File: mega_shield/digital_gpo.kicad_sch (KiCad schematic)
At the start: 26 parts, among them J23 1803277, J24 1803277, Q25 MMBT3904, Q26 MMBT3906, Q27 MMBT3904, Q28 MMBT3906, Q29 AO4486, Q30 AO4486, U26 ADuM1200

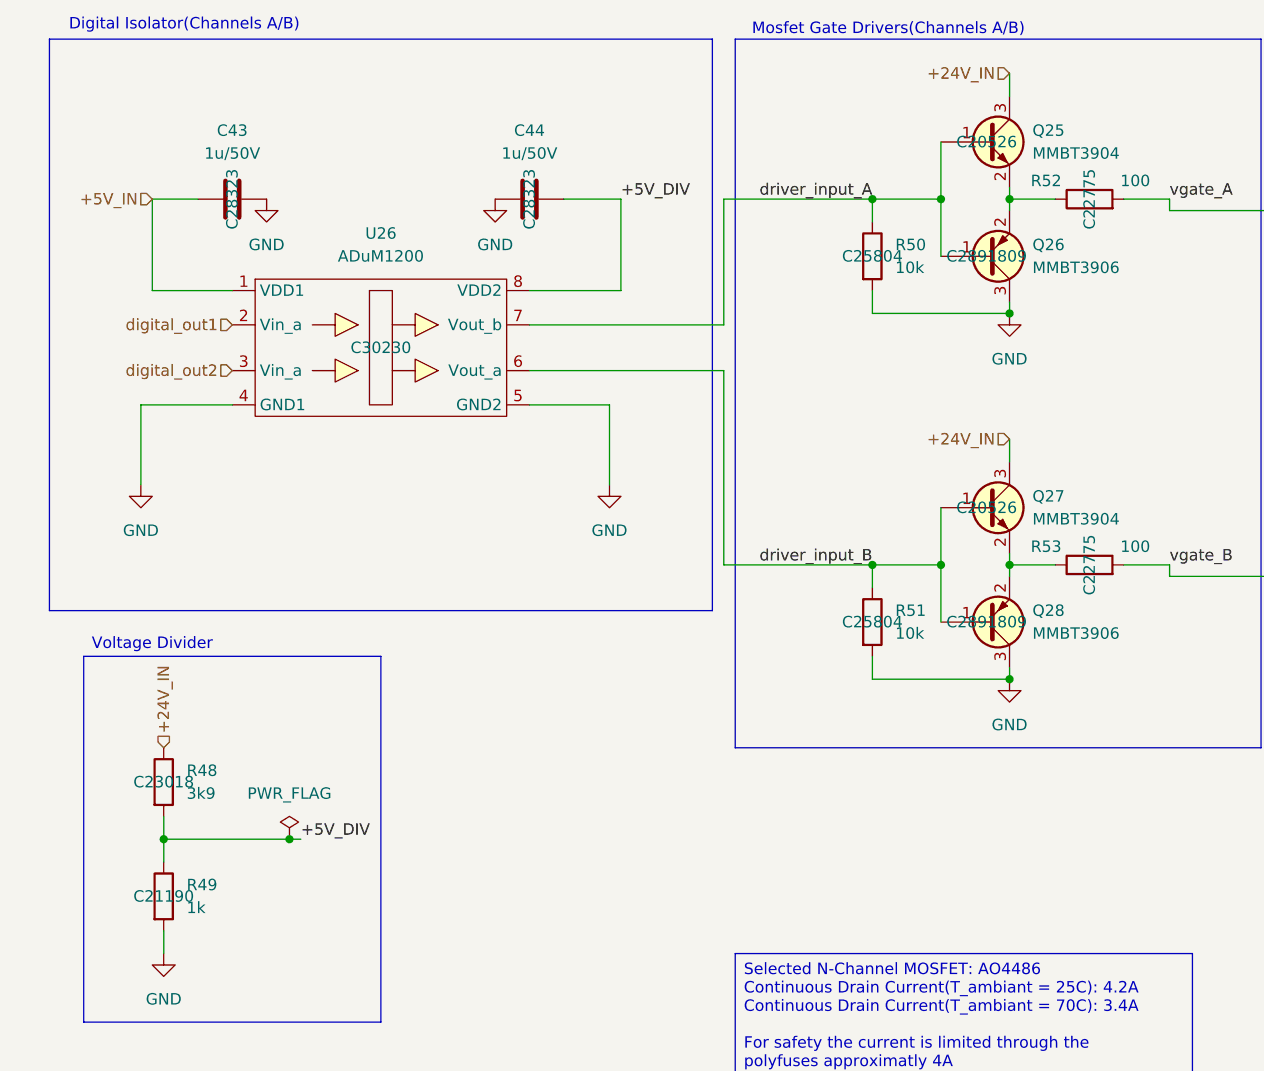
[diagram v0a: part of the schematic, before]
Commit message: mega_shield, updated multiple resistors and added comments.
+ Updated optoisolator resistor value --> 15k for better protection.
+ Changed all resistors to 0805 footprints
+ Swapped out expensive values to standardized E24/E96.
+ Updated jlcpcb numbers for all resistors.
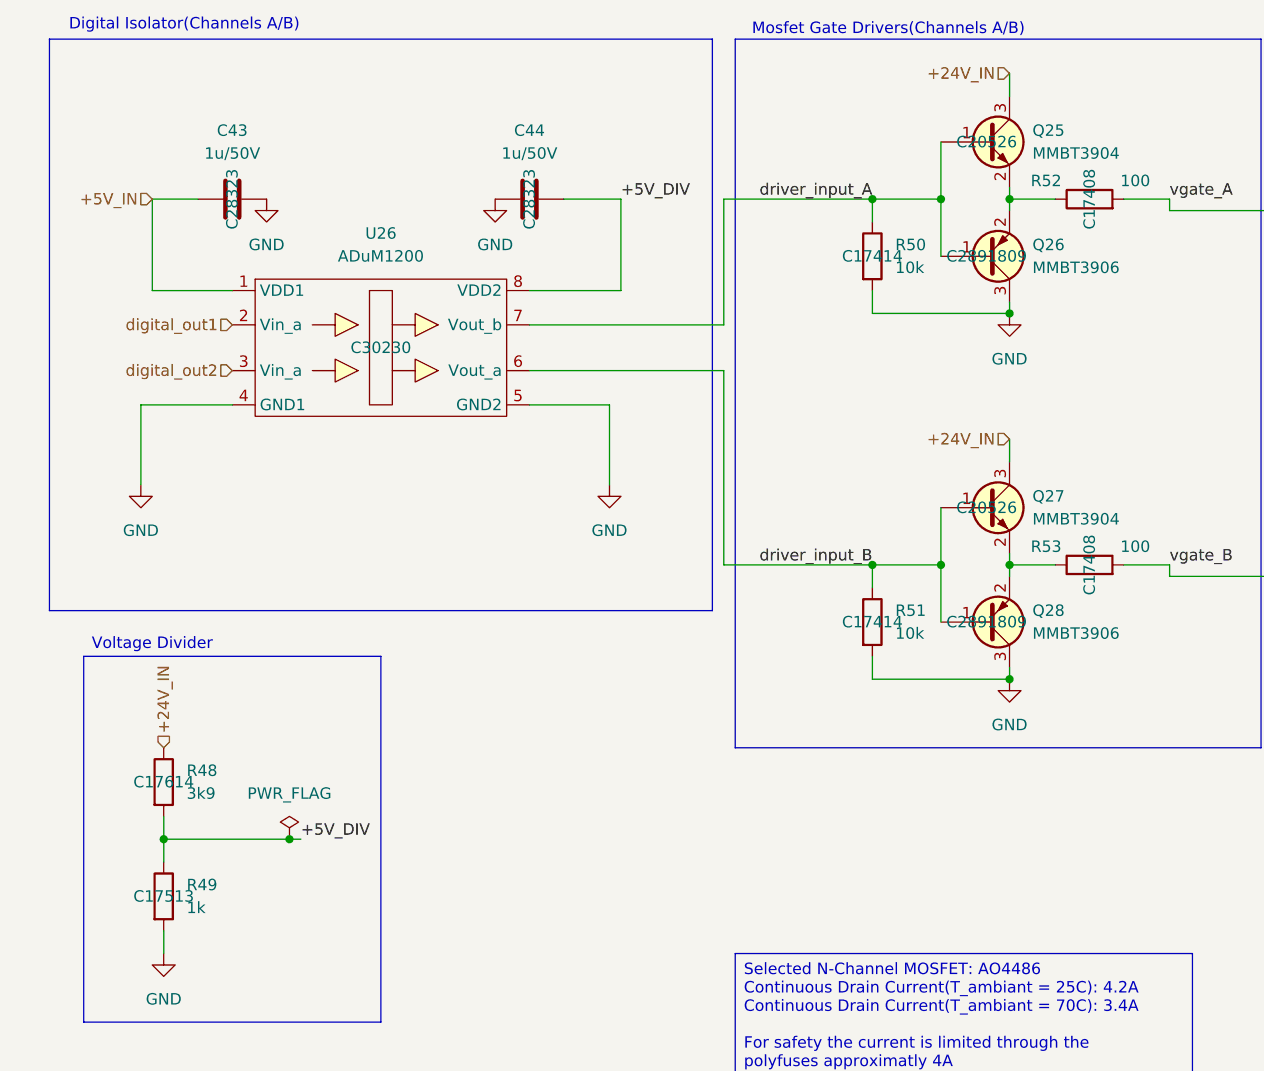
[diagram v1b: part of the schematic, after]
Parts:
- R48: footprint Resistor_SMD:R_0201_0603Metric -> Resistor_SMD:R_0805_2012Metric_Pad1.20x1.40mm_HandSolder; jlcpcb C23018 -> C17614
- R49: footprint Resistor_SMD:R_0201_0603Metric -> Resistor_SMD:R_0805_2012Metric_Pad1.20x1.40mm_HandSolder; jlcpcb C21190 -> C17513
- R50, R51: footprint Resistor_SMD:R_0201_0603Metric -> Resistor_SMD:R_0805_2012Metric_Pad1.20x1.40mm_HandSolder; jlcpcb C25804 -> C17414
- R52, R53: footprint Resistor_SMD:R_0201_0603Metric -> Resistor_SMD:R_0805_2012Metric_Pad1.20x1.40mm_HandSolder; jlcpcb C22775 -> C17408
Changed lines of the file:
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@@
 			)
 		)
-		(property "Footprint" "Resistor_SMD:R_0201_0603Metric"
+		(property "Footprint" "Resistor_SMD:R_0805_2012Metric_Pad1.20x1.40mm_HandSolder"
 			(at 140.97 70.358 90)
 			(effects
@@
 			)
 		)
-		(property "jlcpcb" "C22775"
+		(property "jlcpcb" "C17408"
 			(at 140.97 68.58 0)
 			(effects
@@
 			)
 		)
-		(property "Footprint" "Resistor_SMD:R_0201_0603Metric"
+		(property "Footprint" "Resistor_SMD:R_0805_2012Metric_Pad1.20x1.40mm_HandSolder"
 			(at 115.062 115.57 90)
 			(effects
@@
 			)
 		)
-		(property "jlcpcb" "C25804"
+		(property "jlcpcb" "C17414"
 			(at 116.84 115.57 0)
 			(effects
@@
 			)
 		)
-		(property "Footprint" "Resistor_SMD:R_0201_0603Metric"
+		(property "Footprint" "Resistor_SMD:R_0805_2012Metric_Pad1.20x1.40mm_HandSolder"
 			(at 115.062 74.93 90)
 			(effects
@@
 			)
 		)
-		(property "jlcpcb" "C25804"
+		(property "jlcpcb" "C17414"
 			(at 116.84 74.93 0)
 			(effects
@@
 			)
 		)
-		(property "Footprint" "Resistor_SMD:R_0201_0603Metric"
+		(property "Footprint" "Resistor_SMD:R_0805_2012Metric_Pad1.20x1.40mm_HandSolder"
 			(at 36.322 146.05 90)
 			(effects
@@
 			)
 		)
-		(property "jlcpcb" "C21190"
+		(property "jlcpcb" "C17513"
 			(at 38.1 146.05 0)
 			(effects
@@
 			)
 		)
-		(property "Footprint" "Resistor_SMD:R_0201_0603Metric"
+		(property "Footprint" "Resistor_SMD:R_0805_2012Metric_Pad1.20x1.40mm_HandSolder"
 			(at 140.97 110.998 90)
 			(effects
@@
 			)
 		)
-		(property "jlcpcb" "C22775"
+		(property "jlcpcb" "C17408"
 			(at 140.97 109.22 0)
 			(effects
@@
 			)
 		)
-		(property "Footprint" "Resistor_SMD:R_0201_0603Metric"
+		(property "Footprint" "Resistor_SMD:R_0805_2012Metric_Pad1.20x1.40mm_HandSolder"
 			(at 36.322 133.35 90)
 			(effects
@@
 			)
 		)
-		(property "jlcpcb" "C23018"
+		(property "jlcpcb" "C17614"
 			(at 38.1 133.35 0)
 			(effects
